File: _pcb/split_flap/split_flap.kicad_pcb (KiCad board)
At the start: 2 copper layers, 74 x 74 mm, 13 parts, among them J1 xiao esp32-c3, J2 stepper a4988, J3 ., J4 ., J6 bornier_alimentation_12VDC, J7 Conn_02x05_Odd_Even, U1 LM7805_TO220

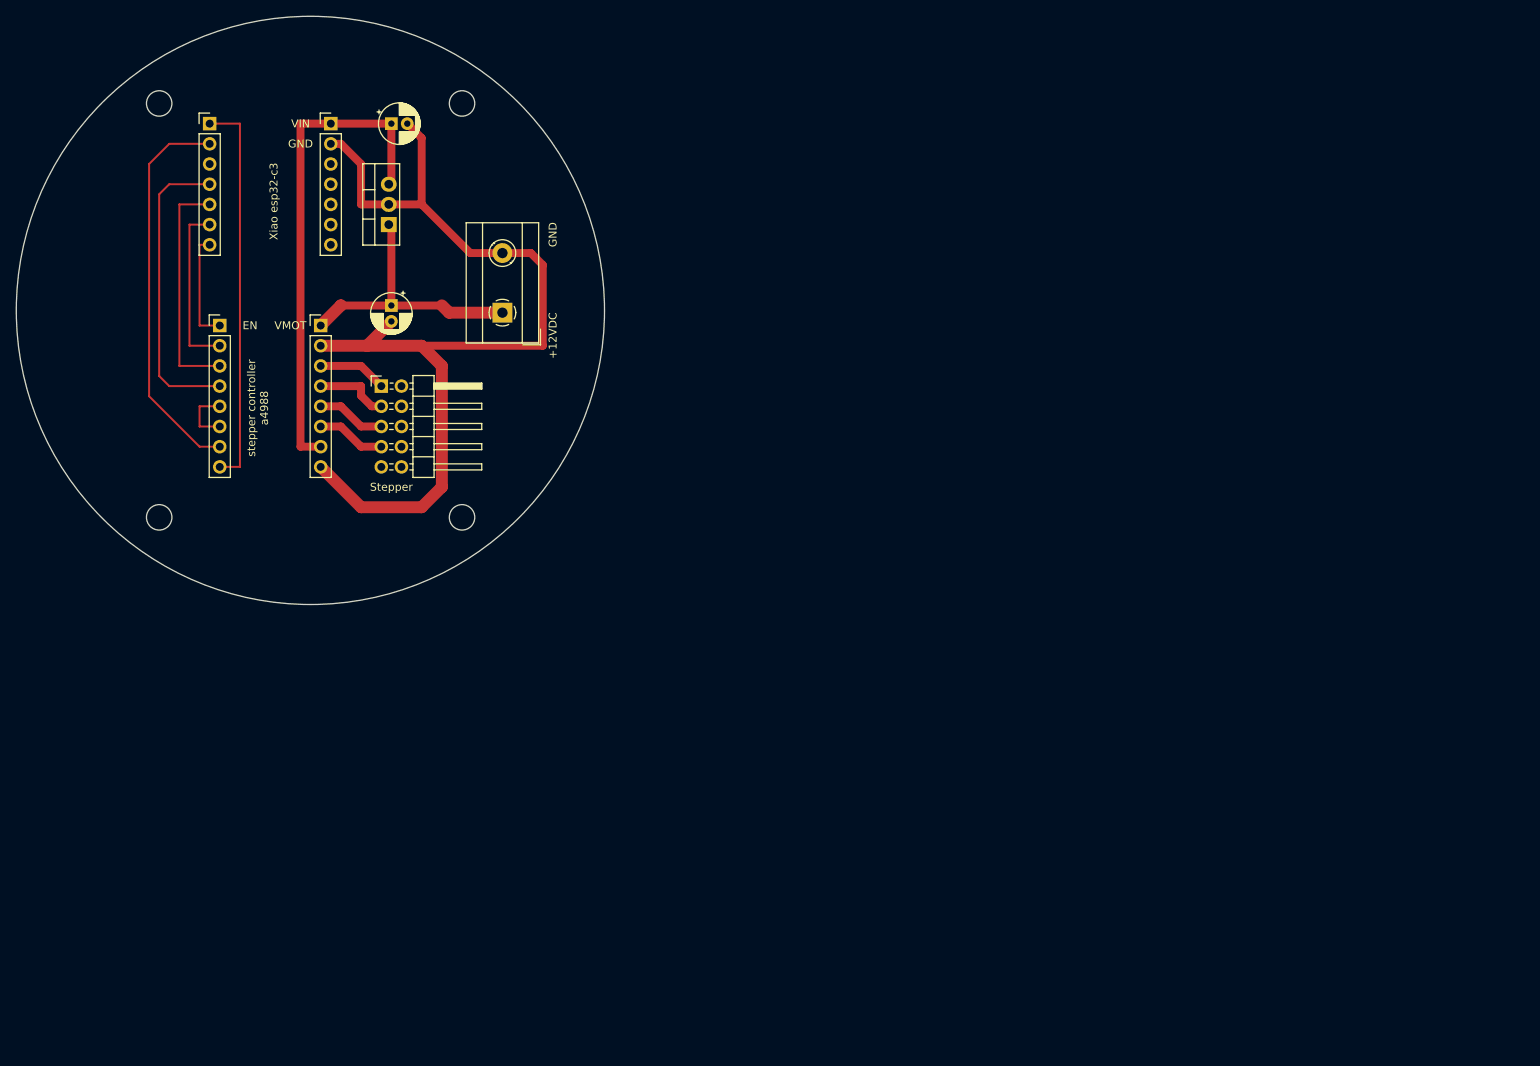
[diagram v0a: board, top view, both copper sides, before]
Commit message: Update split_flap.kicad_pcb
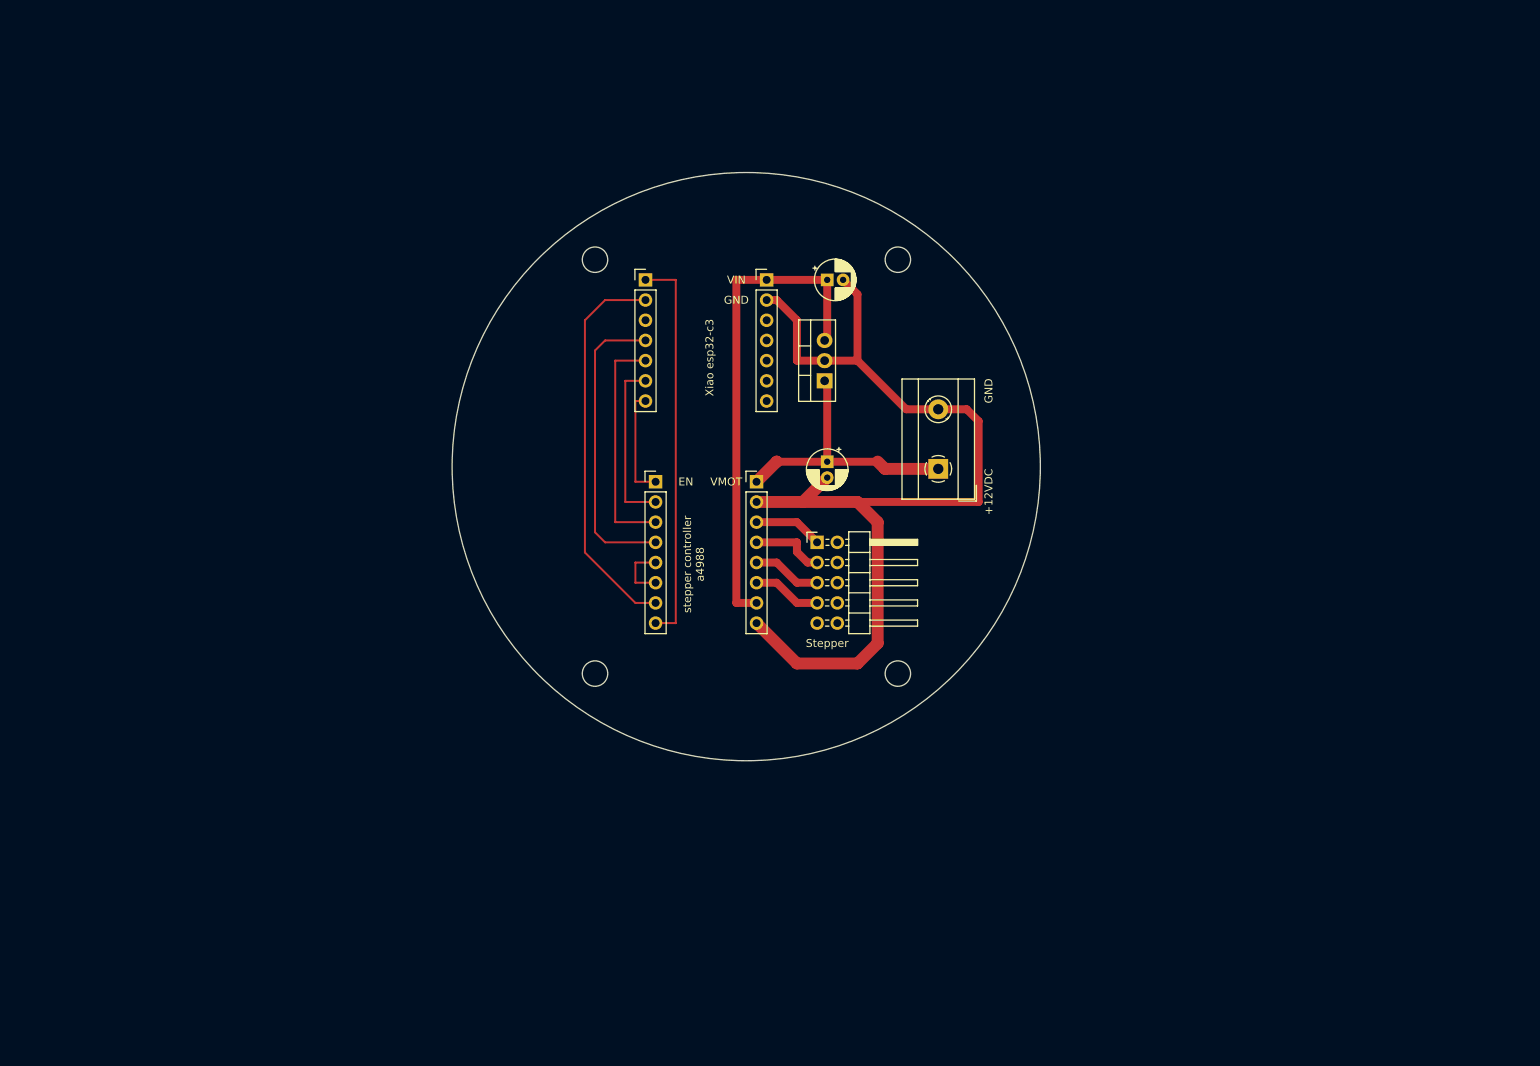
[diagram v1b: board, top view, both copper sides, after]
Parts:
- moved C1 58.2 mm to (152.6, 65.4)
- moved C2 58.2 mm to (152.6, 88.3)
- moved H3 58.2 mm to (123.4, 114.9)
- moved H4 58.2 mm to (123.4, 62.8)
- moved J2 58.2 mm to (131.0, 90.8)
- moved J3 58.2 mm to (145.0, 65.4)
- moved J6 58.2 mm to (166.6, 89.2)
- moved J7 58.2 mm to (151.3, 98.4)
- moved H1 58.2 mm to (161.5, 62.8)
- moved H2 58.2 mm to (161.5, 114.9)
- moved J1 58.2 mm to (129.8, 65.4)
- moved J4 58.2 mm to (143.7, 90.8)
- moved U1 58.2 mm to (152.3, 78.1)

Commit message: backup
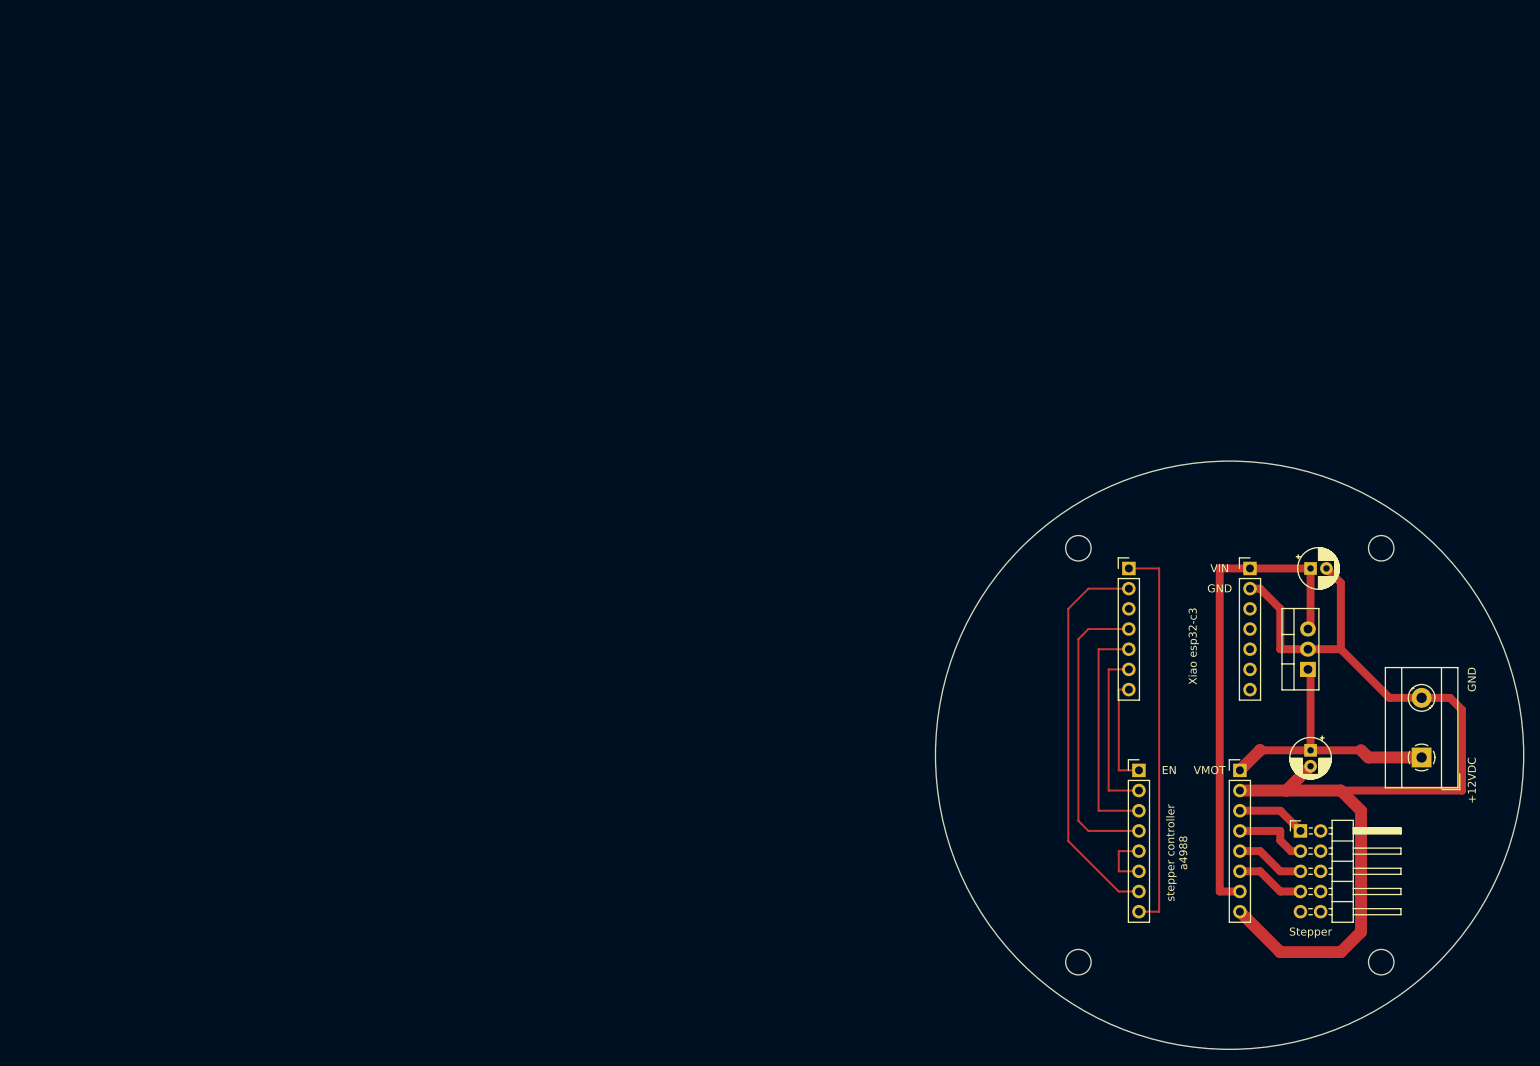
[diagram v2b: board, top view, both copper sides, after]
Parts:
- moved C1 70.8 mm to (213.4, 101.7)
- moved C2 70.8 mm to (213.4, 124.6)
- moved H1 70.8 mm to (222.3, 99.1)
- moved H2 70.8 mm to (222.3, 151.2)
- moved H3 70.8 mm to (184.2, 151.2)
- moved H4 70.8 mm to (184.2, 99.1)
- moved J1 70.8 mm to (190.6, 101.7)
- moved J2 70.8 mm to (191.8, 127.1)
- moved J3 70.8 mm to (205.8, 101.7)
- moved J4 70.8 mm to (204.5, 127.1)
- moved J6 70.8 mm to (227.4, 125.5)
- moved J7 70.8 mm to (212.2, 134.7)
- moved U1 70.8 mm to (213.1, 114.4)

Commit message: A3
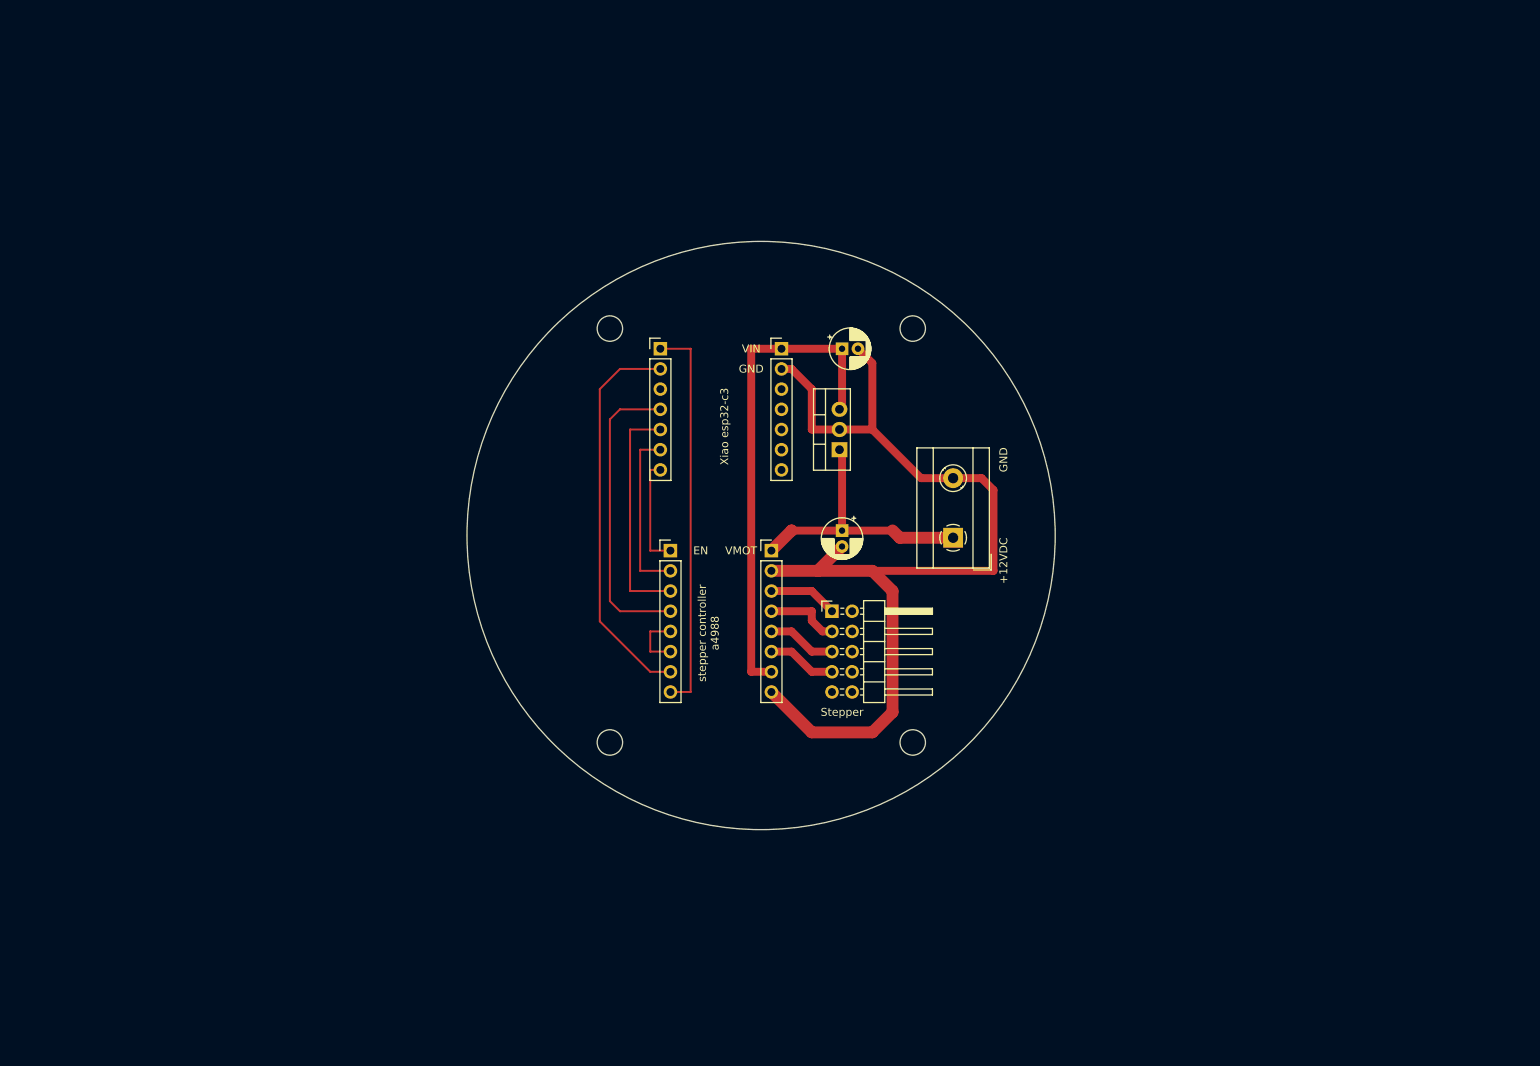
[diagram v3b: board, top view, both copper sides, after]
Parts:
- moved H2 65.1 mm to (163.4, 123.6)
- moved H3 65.1 mm to (125.3, 123.6)
- moved C1 65.1 mm to (154.5, 74.0)
- moved C2 65.1 mm to (154.5, 96.9)
- moved H1 65.1 mm to (163.4, 71.5)
- moved H4 65.1 mm to (125.3, 71.5)
- moved J1 65.1 mm to (131.6, 74.0)
- moved J2 65.1 mm to (132.9, 99.4)
- moved J3 65.1 mm to (146.9, 74.0)
- moved J4 65.1 mm to (145.6, 99.4)
- moved J6 65.1 mm to (168.5, 97.8)
- moved J7 65.1 mm to (153.2, 107.1)
- moved U1 65.1 mm to (154.2, 86.7)
